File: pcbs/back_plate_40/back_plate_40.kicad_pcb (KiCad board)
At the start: 2 copper layers, 131.6 x 107.9 mm, 6 parts

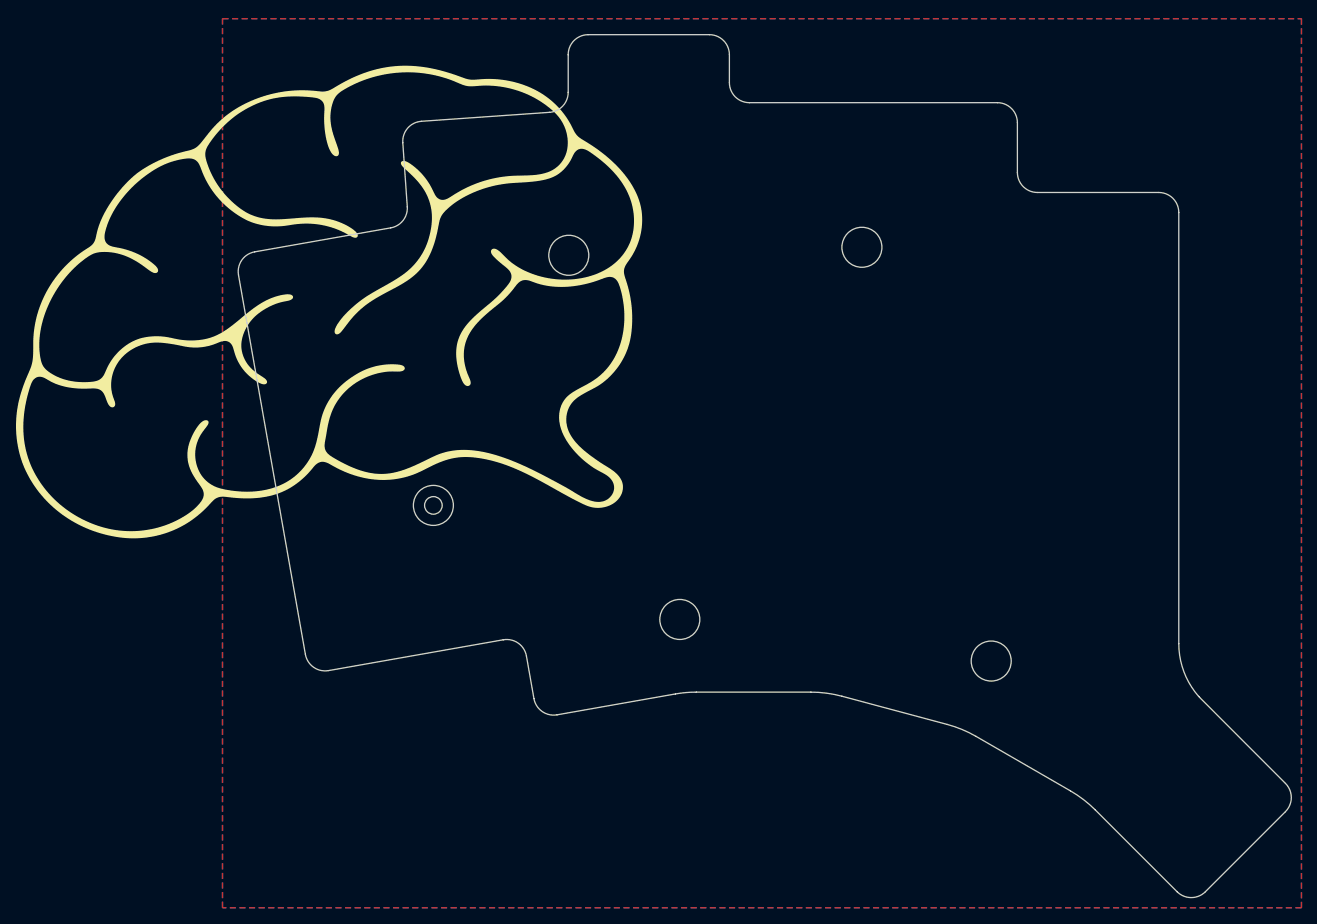
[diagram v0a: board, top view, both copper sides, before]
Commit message: update generated files
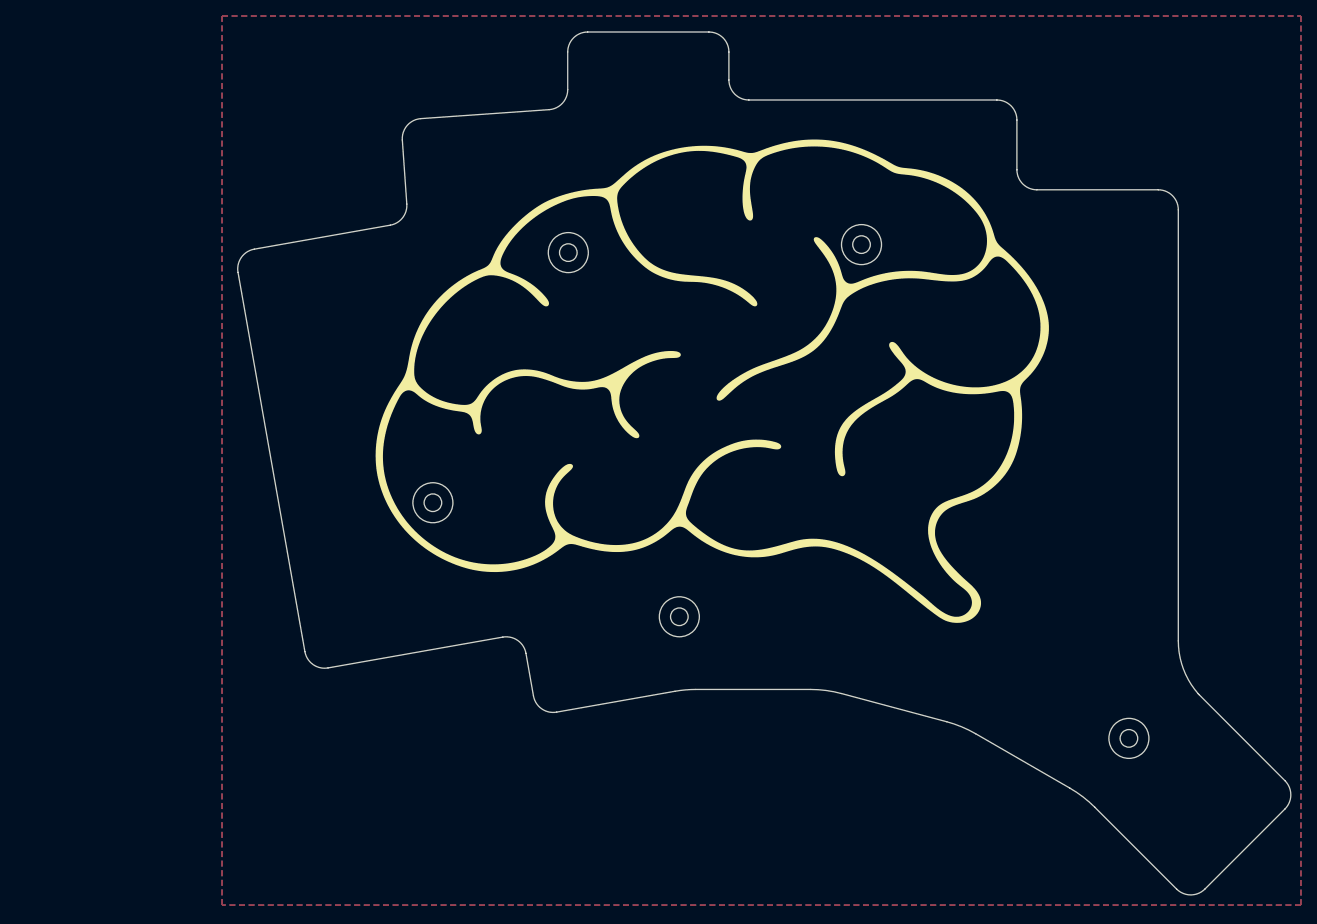
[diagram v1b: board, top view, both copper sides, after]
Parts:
- moved G1 48.7 mm to (108.4, 63.0), turned to 0 degrees
- moved MH3 19.7 mm to (160.5, 107.7), turned to -30 degrees
- moved MH4 0.34 mm to (104.3, 92.5)
- moved MH5 0.34 mm to (73.5, 78.3)
- moved MH1 0.34 mm to (90.4, 47.0)
- moved MH2 0.34 mm to (127.1, 46.0)
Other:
- outline, holes or cut-outs redrawn

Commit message: update generated files
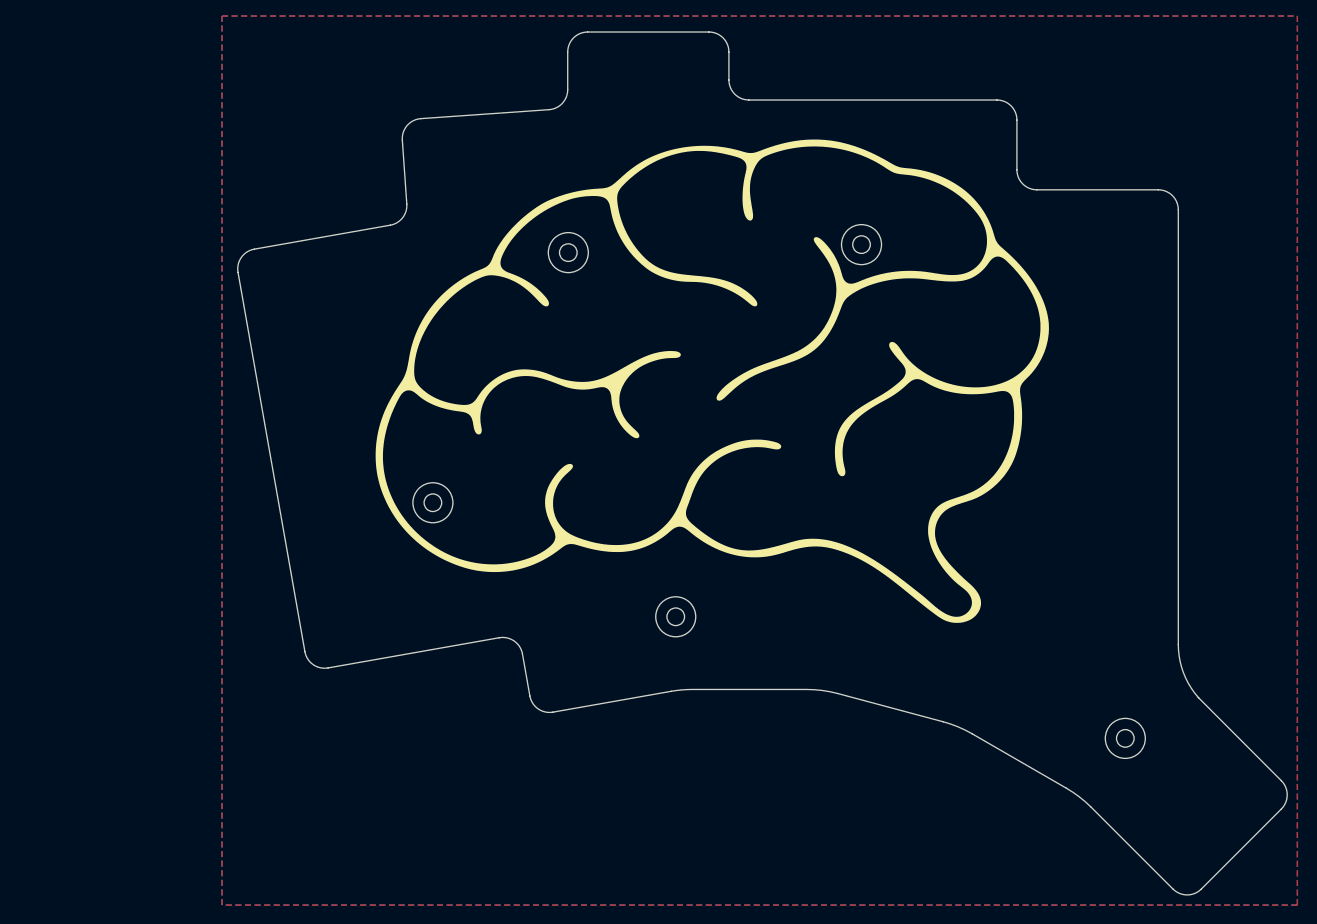
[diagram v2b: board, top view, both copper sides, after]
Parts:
- moved MH3 0.45 mm to (160.0, 107.7)
- moved MH4 0.45 mm to (103.9, 92.5)
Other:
- board size 131.6 x 107.9 mm -> 131.2 x 107.9 mm
